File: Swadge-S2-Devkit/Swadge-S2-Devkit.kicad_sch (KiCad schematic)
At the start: 92 parts, among them J1 LED, J2 Conn_02x10_Odd_Even, J3 Conn_01x05_Male, P1 USB_C_Plug_USB2.0, Q1 Q_PMOS_GSD, SW1 TS-1109S-A-A, SW2 TS-1109S-A-A, SW3 TS-1109S-A-A, SW4 TS-1109S-A-A, SW5 TS-1109S-A-A, SW6 TS-1109S-A-A, SW7 B3FS-4002P, SW8 B3FS-4002P, SW9 SW_SPDT_1825232-1, U1 ESP32-S2-SOLO, U10 GENERIC_LDO_2.8, U11 art_melee_logo, U12 art_select_start, U13 art_squarewavebird, U14 RB017A1505A_Connector, U15 RB0154A1201A, U16 Controller_Shields, U2 RB017A1505A, U3 MT3410, U5 art_xy_buttons, U6 art_20th_logo, U7 art_d_pad, U8 art_eyebrow

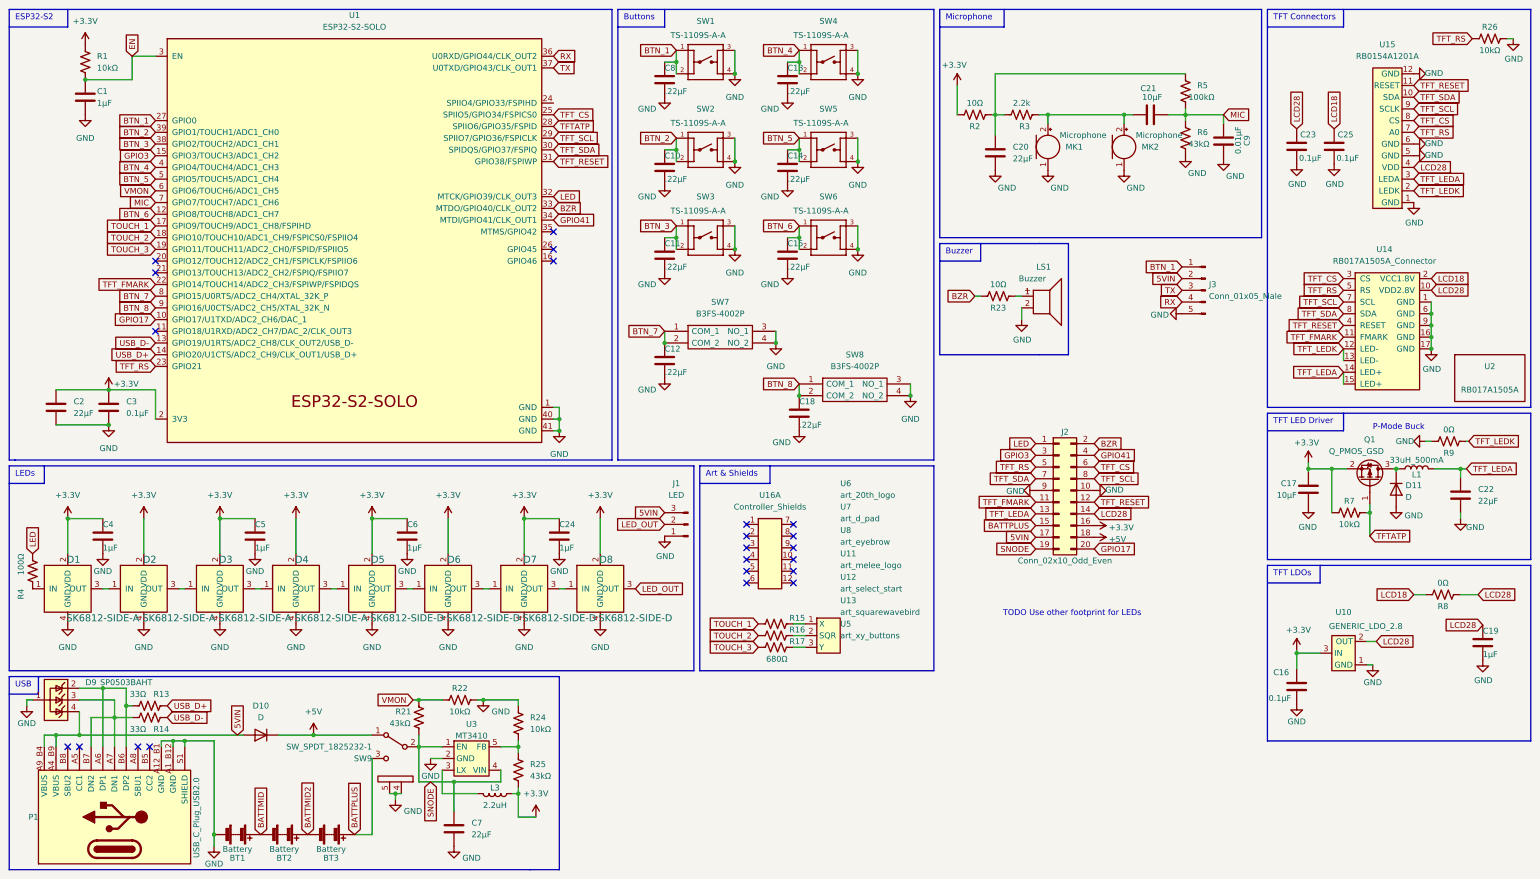
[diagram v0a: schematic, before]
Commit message: Update design, routed.
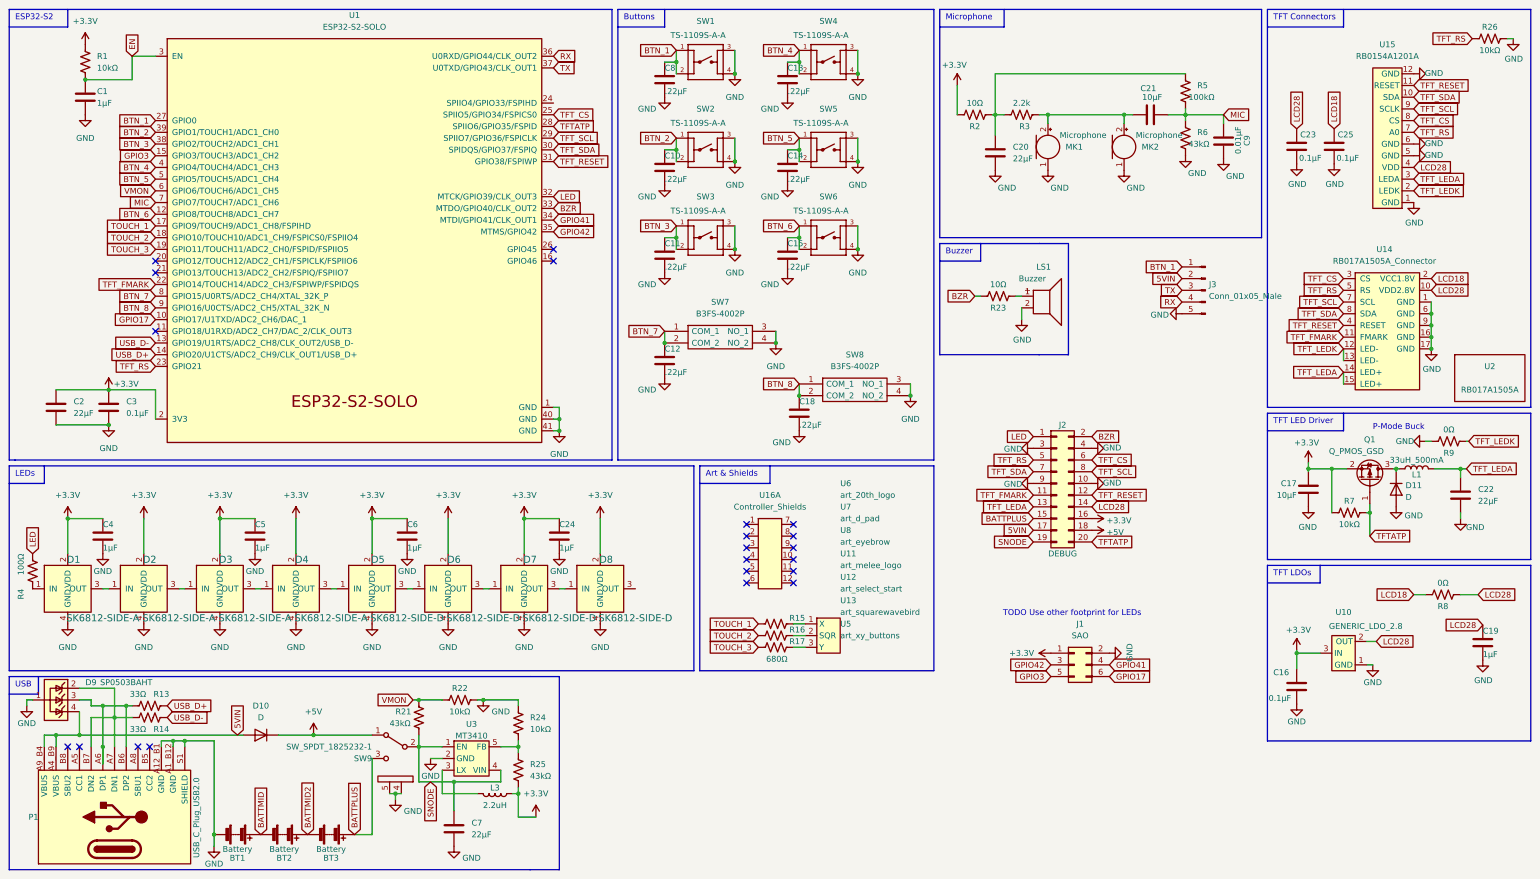
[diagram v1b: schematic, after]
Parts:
- removed J1: LED, Swadge_Parts:PinHeader_1x03_P2.54mm_Vertical, symbol Swadge_Parts:Conn_01x03_Male
- added J1: SAO, Connector_PinSocket_2.54mm:PinSocket_2x03_P2.54mm_Vertical, symbol Connector_Generic:Conn_02x03_Odd_Even
- J2: value Conn_02x10_Odd_Even -> DEBUG
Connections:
- net +3V3: now also J1.1 (Pin_1)
- net GND: now also J2.3 (Pin_3), J2.4 (Pin_4), J1.2 (Pin_2)
- net GPIO17: now also J1.6 (Pin_6); no longer J2.20 (Pin_20)
- net GPIO3: now also J1.5 (Pin_5); no longer J2.3 (Pin_3)
- net GPIO41: now also J1.4 (Pin_4); no longer J2.4 (Pin_4)
- net TFTATP: now also J2.20 (Pin_20)
- net at P1.A6 (DP1), P1.B6 (DP2), R13.2: now also D9.3 (K); no longer D9.2 (K)
- net GPIO42: now reaches U1.35 (MTMS/GPIO42)
- net GPIO42: now also J1.3 (Pin_3)
- net at P1.A7 (DN1), P1.B7 (DN2), R14.2: now also D9.2 (K); no longer D9.3 (K)
- net LED_OUT: no longer names the net of D8.3 (OUT)
- no-connect marks 22 -> 21
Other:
- moved on the sheet: J2
